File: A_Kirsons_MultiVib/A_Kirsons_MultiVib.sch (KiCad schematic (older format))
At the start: 11 parts

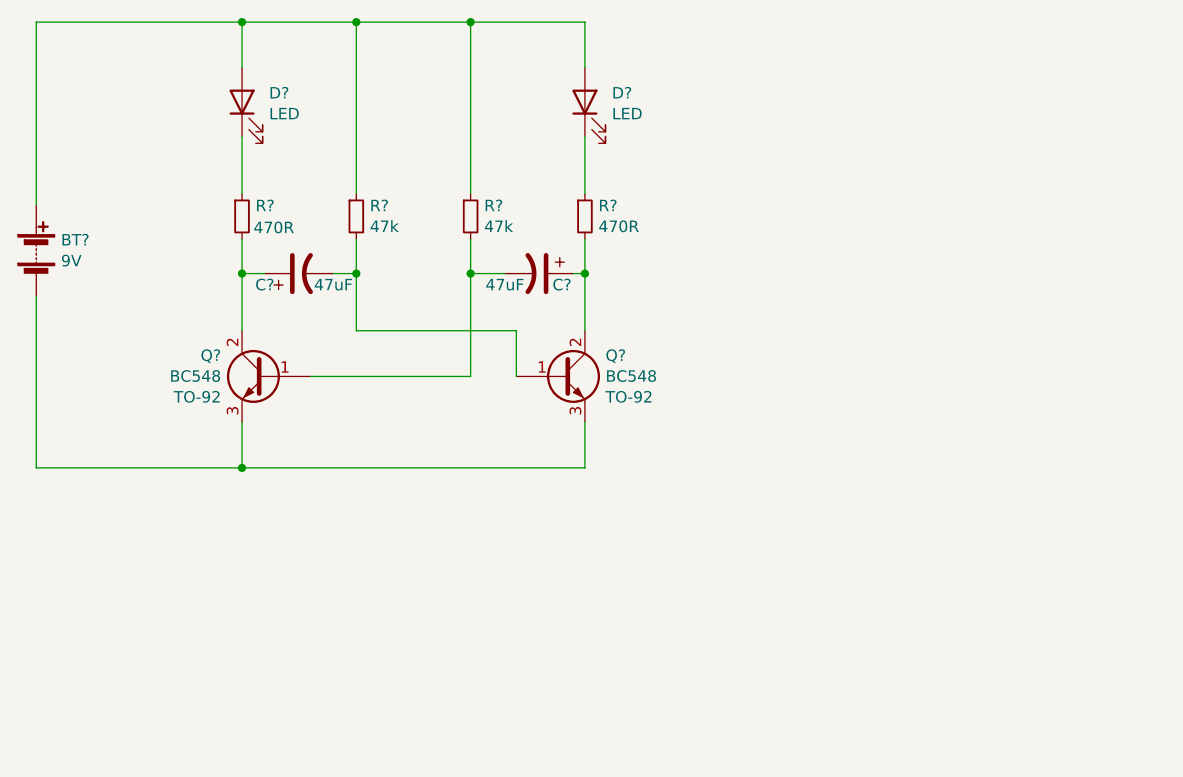
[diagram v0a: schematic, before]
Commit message: A_Kirsons_MultiVib update to test GitHub Repo
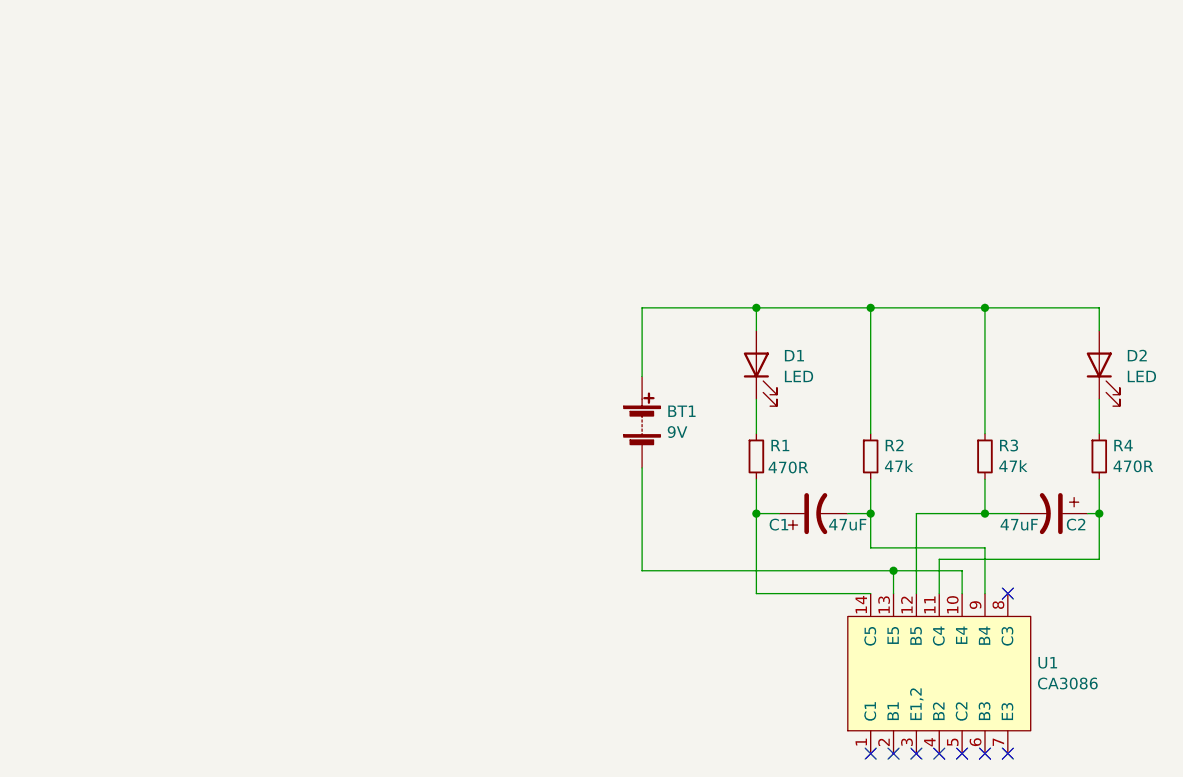
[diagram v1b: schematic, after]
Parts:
- removed BT?: 9V, symbol Device:Battery
- removed C? (x2): 47uF, symbol Device:CP1
- removed D? (x2): LED, symbol Device:LED
- removed Q? (x2): BC548, symbol Device:Q_NPN_BCE
- removed R? (x2): 470R, symbol Device:R_Small
- removed R? (x2): 47k, symbol Device:R_Small
- added BT1: 9V, symbol Device:Battery
- added C1, C2: 47uF, symbol Device:CP1
- added D1, D2: LED, symbol Device:LED
- added R1, R4: 470R, symbol Device:R_Small
- added R2, R3: 47k, symbol Device:R_Small
- added U1: CA3086, symbol New_Library:CA3086
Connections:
- new net: BT1.2 (-), U1.10 (E4), U1.13 (E5)
- new net: C2.1, R4.2, U1.11 (C4)
- new net: C2.2, R3.2, U1.12 (B5)
- new net: C1.1, R1.2, U1.14 (C5)
- new net: C1.2, R2.2, U1.9 (B4)
- new net: D1.1 (K), R1.1
- new net: BT1.1 (+), D1.2 (A), D2.2 (A), R2.1, R3.1
- new net: D2.1 (K), R4.1
- no-connect marks 0 -> 8
